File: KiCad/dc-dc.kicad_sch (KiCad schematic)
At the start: 60 parts, among them Q1 NMOS, Q2 NMOS, Q3 NMOS, Q4 NMOS, U3 LT8390xFE

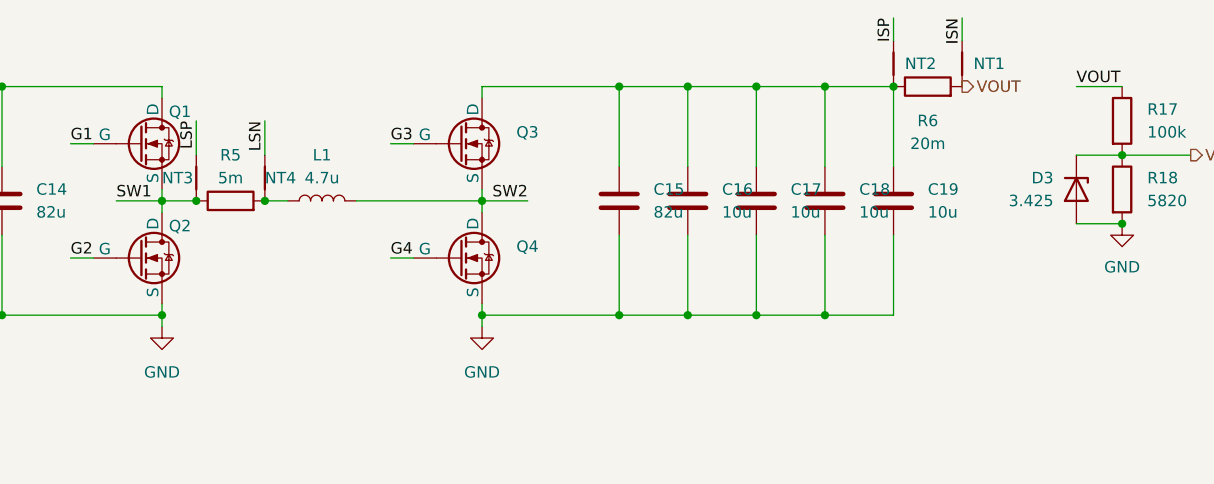
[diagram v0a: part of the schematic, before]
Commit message: new layout
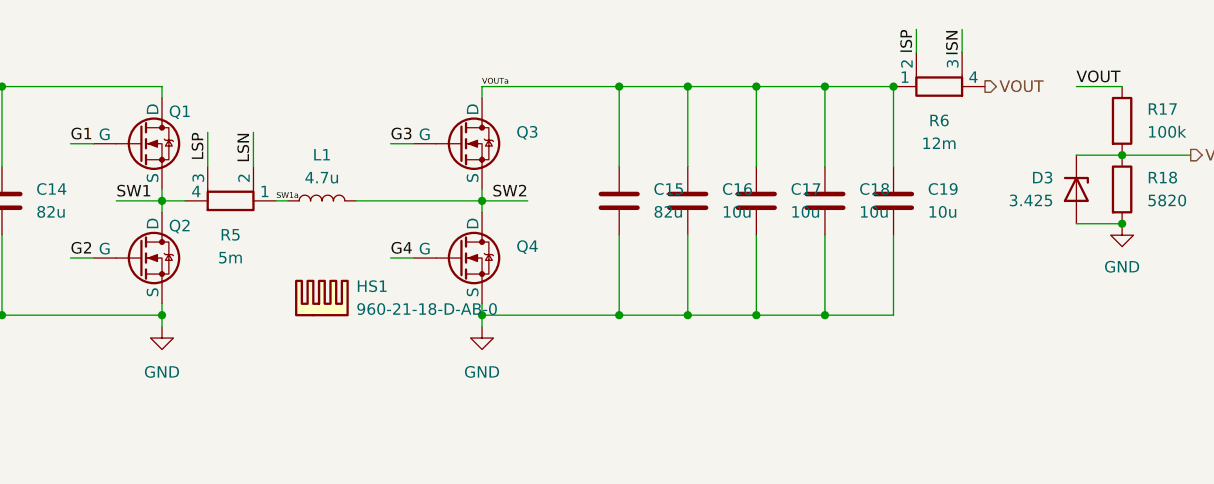
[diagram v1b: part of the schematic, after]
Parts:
- removed NT1, NT2, NT3, NT4: NetTie_2, symbol Device:NetTie_2
- removed R5: 5m, Resistor_SMD:R_1206_3216Metric, symbol Device:R
- removed R6: 20m, Resistor_SMD:R_1206_3216Metric, symbol Device:R
- added HS1: 960-21-18-D-AB-0, Library:960-21-xx-D, symbol Mechanical:Heatsink
- added R5: 5m, Resistor_SMD:R_Shunt_Ohmite_LVK12, symbol Device:R_Shunt
- added R6: 12m, Resistor_SMD:R_Shunt_Ohmite_LVK12, symbol Device:R_Shunt
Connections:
- net ISN: now also R6.3
- net ISP: now also R6.2
- net LSN: now also R5.2
- net LSP: now also R5.3
- net SW1: now also R5.4
- net VOUT: now also R6.4
- net VOUTa: now reaches C15.1, C16.1, C17.1, C18.1, C19.1, Q3.1 (D)
- net VOUTa: now also R6.1
- net SW1a: now reaches L1.1
- net SW1a: now also R5.1
